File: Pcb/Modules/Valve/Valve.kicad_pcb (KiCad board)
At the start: 2 copper layers, 53.3 x 45.7 mm, 19 parts, among them CON1 Valve1, CON2 Valve3, CON3 Power, CON4 Valve2, CON5 Valve4, J1 JACK_RJ45, P1 Servo1, P2 Servo2, Q1 Q_NMOS_GSD, Q2 Q_NMOS_GSD, Q3 Q_NMOS_GSD, Q4 Q_NMOS_GSD

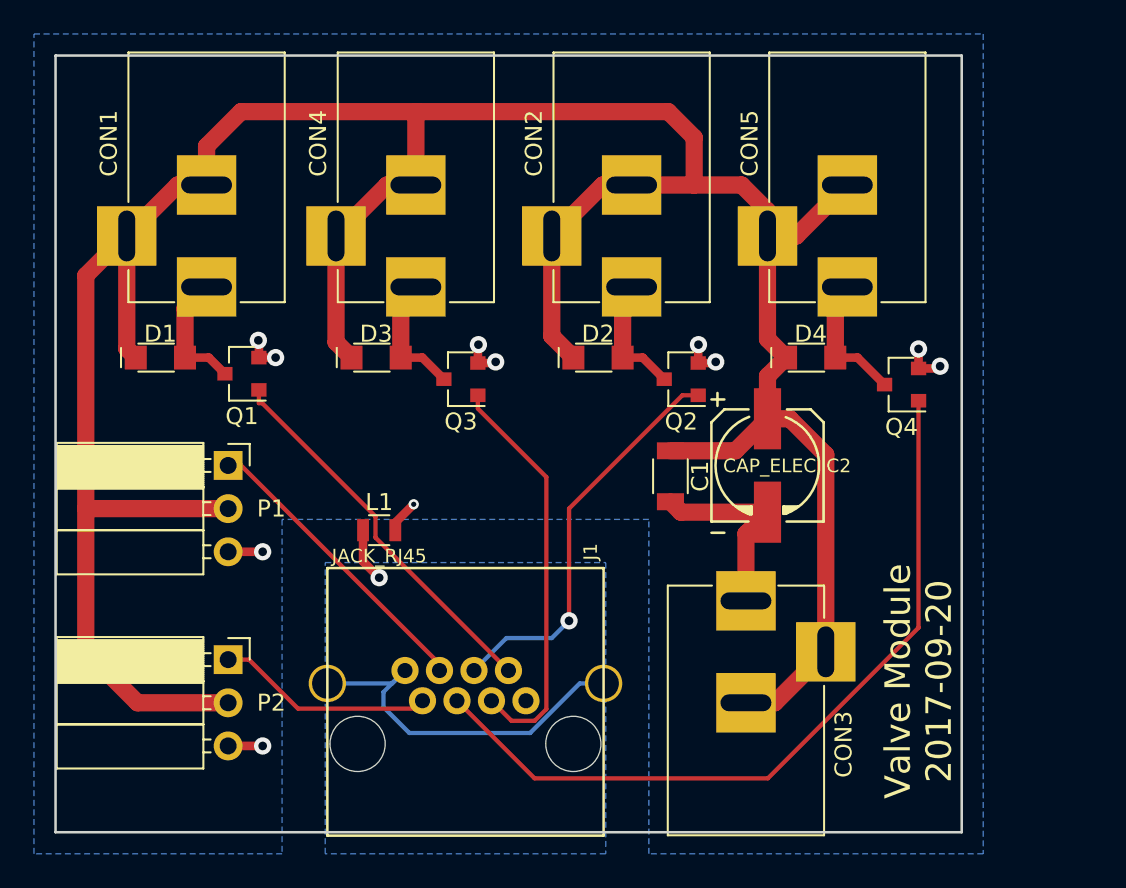
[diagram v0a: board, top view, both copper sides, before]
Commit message: Update Valve module
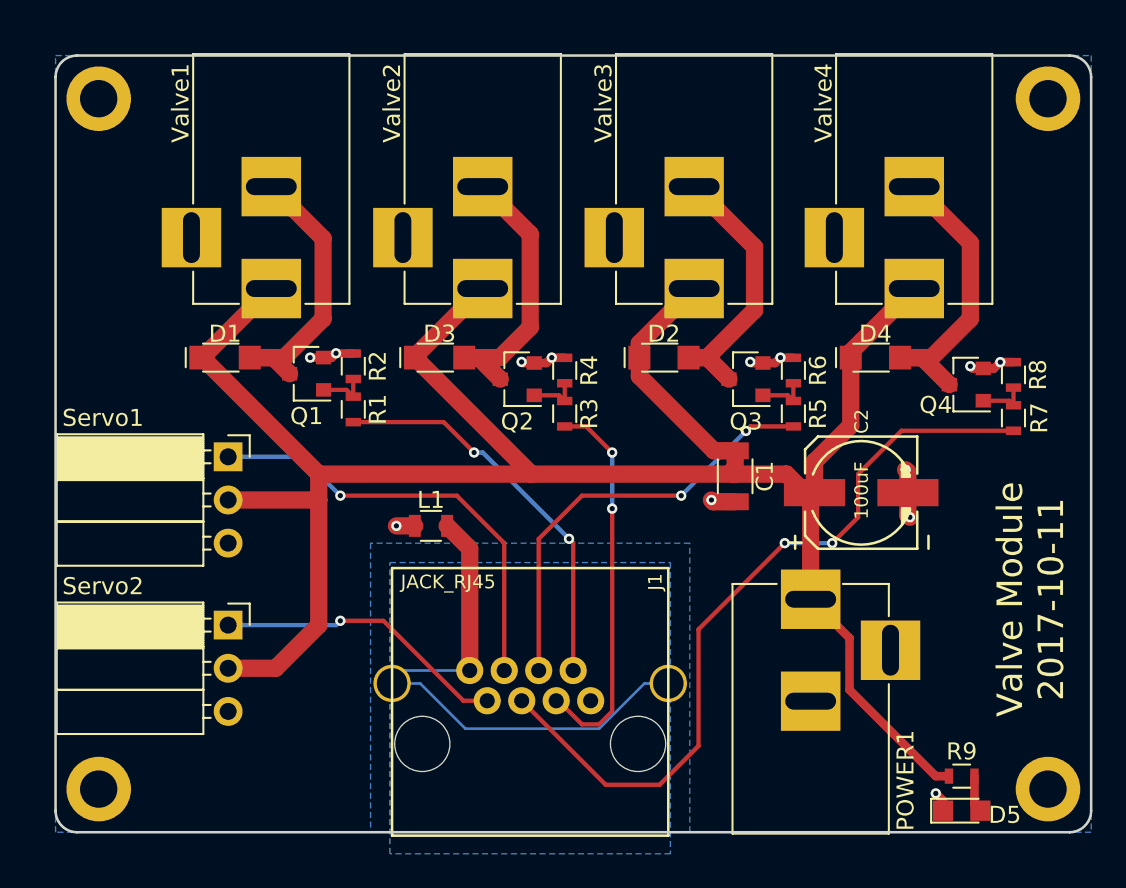
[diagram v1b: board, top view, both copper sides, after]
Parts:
- removed CON1: Valve1, Connectors:BARREL_JACK
- removed CON2: Valve3, Connectors:BARREL_JACK
- removed CON3: Power, Connectors:BARREL_JACK
- removed CON4: Valve2, Connectors:BARREL_JACK
- removed CON5: Valve4, Connectors:BARREL_JACK
- added D5: LED, LEDs:LED_0805, F.Cu at (78.7, 69.8)
- added POWER1: Power, Connectors:BARREL_JACK, F.Cu at (69.8, 57.4)
- added R1: 1K, Resistors_SMD:R_0603, F.Cu at (42.9, 46.2)
- added R2: 10K, Resistors_SMD:R_0603, F.Cu at (42.9, 43.7)
- added R3: 1K, Resistors_SMD:R_0603, F.Cu at (55.4, 46.5)
- added R4: 10K, Resistors_SMD:R_0603, F.Cu at (55.4, 43.9)
- added R5: 1K, Resistors_SMD:R_0603, F.Cu at (68.8, 46.5)
- added R6: 10K, Resistors_SMD:R_0603, F.Cu at (68.8, 43.9)
- added R7: 1K, Resistors_SMD:R_0603, F.Cu at (81.8, 46.7)
- added R8: 10K, Resistors_SMD:R_0603, F.Cu at (81.8, 44.2)
- added R9: 1K, Resistors_SMD:R_0603, F.Cu at (78.7, 67.8)
- added Valve1: Valve1, Connectors:BARREL_JACK, F.Cu at (38.1, 39.1)
- added Valve2: Valve2, Connectors:BARREL_JACK, F.Cu at (50.5, 39.1)
- added Valve3: Valve3, Connectors:BARREL_JACK, F.Cu at (63.0, 39.1)
- added Valve4: Valve4, Connectors:BARREL_JACK, F.Cu at (75.9, 39.1)
- added X1: HOLE, Mounting_Holes:MountingHole_2.2mm_M2_ISO14580_Pad, F.Cu at (27.9, 27.9)
- added X2: HOLE, Mounting_Holes:MountingHole_2.2mm_M2_ISO14580_Pad, F.Cu at (83.8, 27.9)
- added X3: HOLE, Mounting_Holes:MountingHole_2.2mm_M2_ISO14580_Pad, F.Cu at (27.9, 68.6)
- added X4: HOLE, Mounting_Holes:MountingHole_2.2mm_M2_ISO14580_Pad, F.Cu at (83.8, 68.6)
- C1: value C -> 10uF
- C2: value CAP_ELEC -> 100uF
- moved Q3 16.8 mm to (66.0, 44.5)
- moved Q2 9.65 mm to (52.6, 44.5)
- moved C2 5.74 mm to (72.8, 51.1), turned to 180 degrees
- moved D2 3.88 mm to (61.2, 43.2)
- moved C1 3.81 mm to (65.4, 50.2)
- moved D1 3.81 mm to (35.4, 43.2)
- moved D4 3.81 mm to (73.7, 43.2)
- moved J1 3.81 mm to (53.3, 63.5)
- moved Q1 3.81 mm to (40.2, 44.1)
- moved Q4 3.81 mm to (79.0, 44.8)
- moved D3 3.74 mm to (48.0, 43.2)
- moved L1 3.06 mm to (47.5, 53.1), turned to 180 degrees
- moved Servo2 2.03 mm to (35.6, 58.9)
- moved Servo1 0.51 mm to (35.6, 49.0)
- renumbered P1 to Servo1, P2 to Servo2
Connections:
- D2 pad 2: Net-(CON2-Pad1) -> Net-(D2-Pad2)
- D3 pad 2: Net-(CON4-Pad1) -> Net-(D3-Pad2)
- Q1 pad 1: /Valve1 -> Net-(Q1-Pad1)
- Q2 pad 1: /Valve3 -> Net-(Q2-Pad1)
- Q2 pad 3: Net-(CON2-Pad1) -> Net-(D3-Pad2)
- Q3 pad 1: /Valve2 -> Net-(Q3-Pad1)
- Q3 pad 3: Net-(CON4-Pad1) -> Net-(D2-Pad2)
- Q4 pad 1: /Valve4 -> Net-(Q4-Pad1)
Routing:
- net +12V: track 179.7 -> 132.3 mm
- net Net-(D3-Pad2): track 0.00 -> 16.7 mm
- net Net-(D2-Pad2): track 0.00 -> 16.7 mm
- net Net-(D4-Pad2): track 8.01 -> 17.8 mm
- net Net-(D1-Pad2): track 7.43 -> 17.0 mm
- net GND: track 26.6 -> 17.5 mm, vias 11 -> 13
- net /Servo1: track 17.8 -> 25.9 mm, vias 0 -> 1
- net Net-(CON4-Pad1): track 7.59 -> 0.00 mm
- net Net-(CON2-Pad1): track 7.36 -> 0.00 mm
- net Net-(J1-Pad8): track 25.5 -> 32.4 mm, vias 1 -> 0
- net /Servo2: track 12.8 -> 17.3 mm, vias 0 -> 1
- net Net-(Q2-Pad1): track 0.00 -> 2.97 mm
- net Net-(Q3-Pad1): track 0.00 -> 2.97 mm
- net Net-(Q1-Pad1): track 0.00 -> 2.95 mm
- net Net-(Q4-Pad1): track 0.00 -> 2.93 mm
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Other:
- board size 53.3 x 45.7 mm -> 61 x 45.7 mm
- rule trace_min: 0.2 -> 0.1524
- board text added: "Valve Module 2017-10-11"
- board text removed: "Valve Module 2017-09-20"
